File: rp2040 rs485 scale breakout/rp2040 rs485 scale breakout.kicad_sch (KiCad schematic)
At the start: 59 parts, among them J1 main i2c, J10 i2c 3, J11 i2c 4, J12 i2c 2, J13 i2c 0, J14 i2c 1, J2 ESDU5V0H4, J3 rs485, J4 Conn_01x01, J5 i2c pullups, J6 qwiic from pro micro, J7 i2c 5, J8 i2c 6, J9 i2c 7, U1 MAX487E, U2 ProMicro_2040, U3 PCA9548ADW

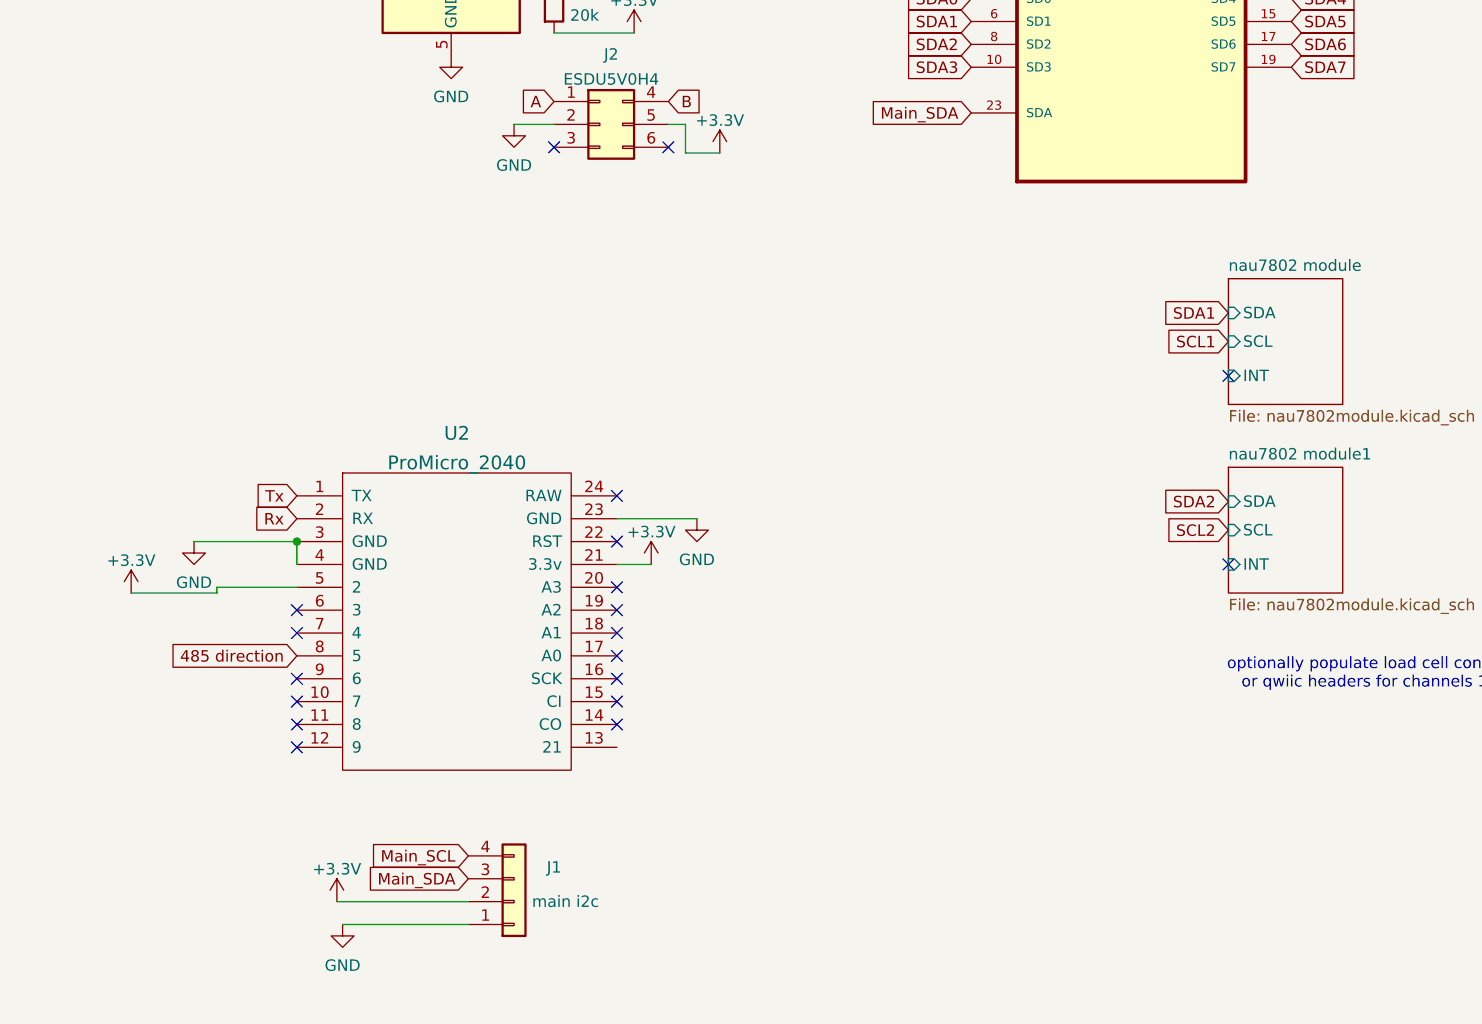
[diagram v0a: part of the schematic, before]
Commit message: motor driver and scale pcb gerbers
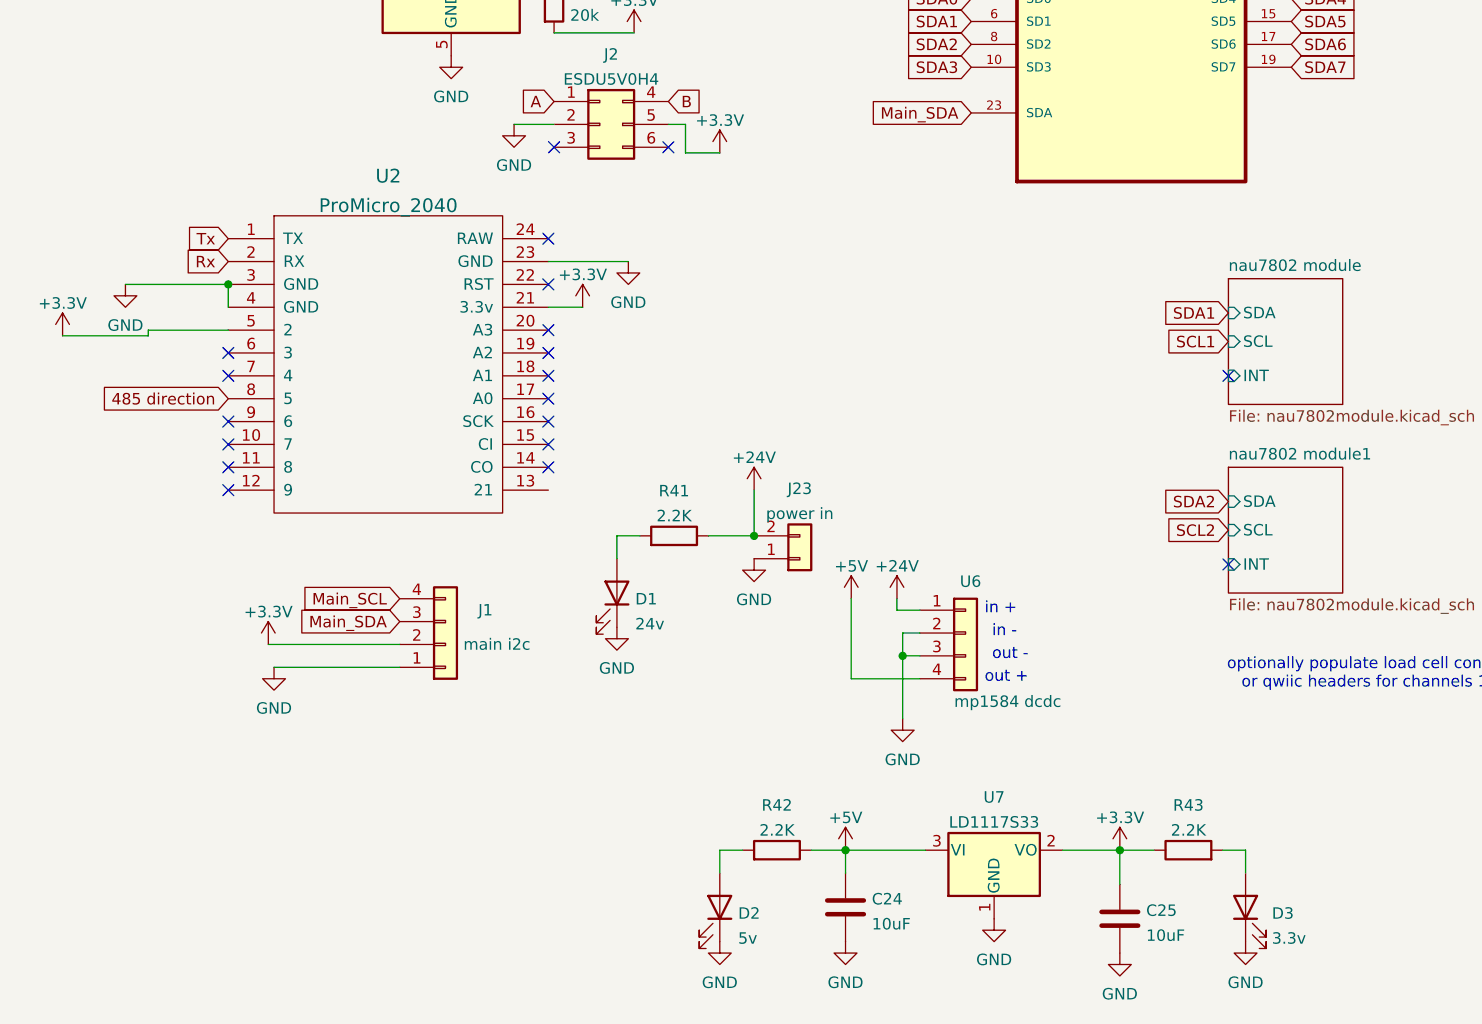
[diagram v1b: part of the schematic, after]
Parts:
- added C24, C25: 10uF, Capacitor_SMD:C_1206_3216Metric, symbol Device:C
- added D1: 24v, LED_SMD:LED_0603_1608Metric, symbol Device:LED
- added D2: 5v, LED_SMD:LED_0603_1608Metric, symbol Device:LED
- added D3: 3.3v, LED_SMD:LED_0603_1608Metric, symbol Device:LED
- added J23: power in, TerminalBlock_Phoenix:TerminalBlock_Phoenix_MKDS-1,5-2_1x02_P5.00mm_Horizontal, symbol Connector_Generic:Conn_01x02
- added R41, R42, R43: 2.2K, Resistor_SMD:R_0603_1608Metric, symbol Device:R
- added U6: mp1584 dcdc, Evan's misc parts:MP1584_buck_module, symbol Connector_Generic:Conn_01x04
- added U7: LD1117S33, Package_TO_SOT_SMD:SOT-223-3_TabPin2, symbol Regulator_Linear:LD1117S33TR_SOT223
- U3: footprint Evan's misc parts:SOIC127P1030X265-24N -> Package_SO:TSSOP-24_4.4x7.8mm_P0.65mm
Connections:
- net +3V3: now also C25.1, R43.1, U7.2 (VO)
- net GND: now also C24.2, C25.2, D1.1 (K), D2.1 (K), D3.1 (K), J23.1 (Pin_1), U6.2 (Pin_2), U6.3 (Pin_3), U7.1 (GND)
- new net: D1.2 (A), R41.2
- new net: D2.2 (A), R42.2
- new net: D3.2 (A), R43.2
- new net +24V: J23.2 (Pin_2), R41.1, U6.1 (Pin_1)
- new net +5V: C24.1, R42.1, U6.4 (Pin_4), U7.3 (VI)
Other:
- note added: "in +"
- note added: "in -"
- note added: "out +"
- note added: "out -"
- moved on the sheet: J1, U2
